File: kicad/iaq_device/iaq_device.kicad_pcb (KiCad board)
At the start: 2 copper layers, 78.2 x 43.2 mm, 18 parts, among them J1 External Pins, SW1 B3S-1000, SW2 CO2 CAL, U2 PMS7003, U3 SSD1306, U4 BME280, U5 MH-Z19, U6 SGP30, U7 TSL2561T

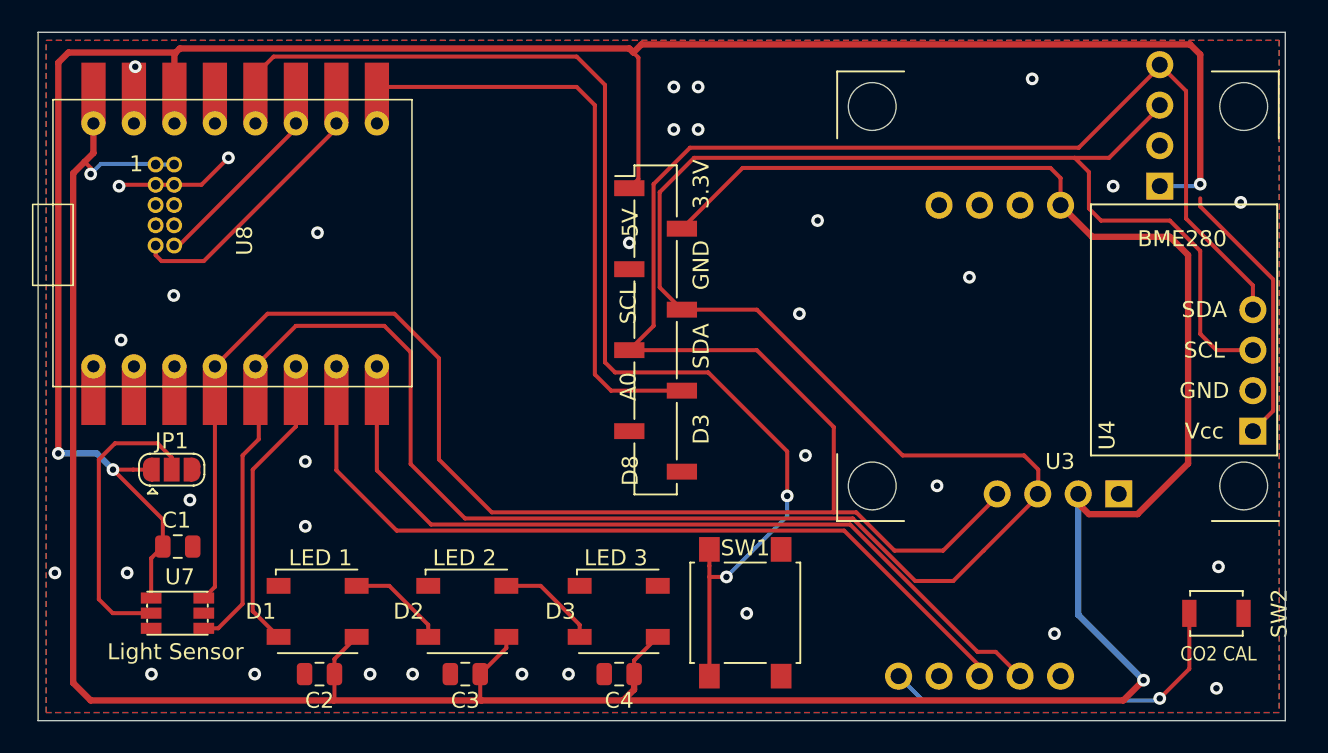
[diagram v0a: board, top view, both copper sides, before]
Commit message: v2.0 of the C3 PCB files
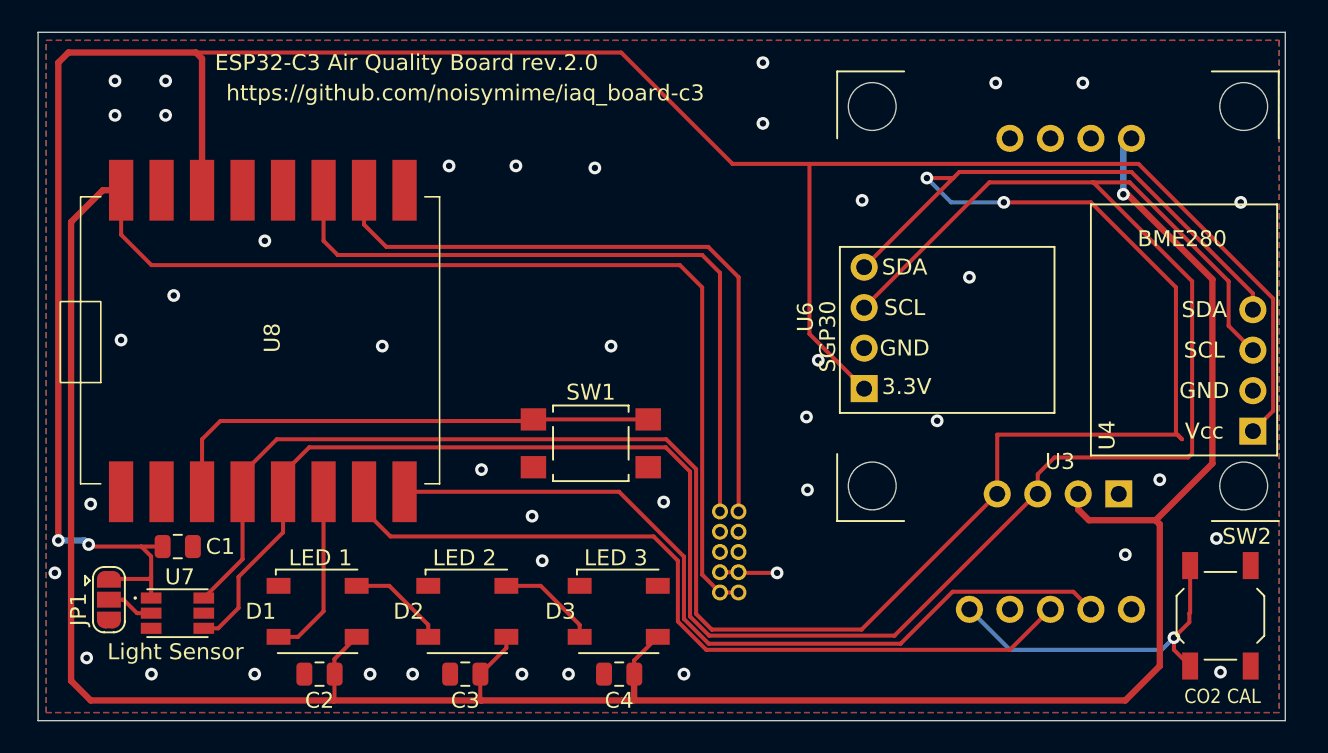
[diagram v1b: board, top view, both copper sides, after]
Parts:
- removed J1: External Pins, Connector_PinSocket_2.54mm:PinSocket_1x08_P2.54mm_Vertical_SMD_Pin1Left
- SW1: value B3S-1000 -> SEL; footprint Nikolay Library:SW_SPST_B3S-1000 -> Button_Switch_SMD:SW_SPST_TL3305B
- SW2: footprint Button_Switch_SMD:SW_SPST_B3U-1000P -> Button_Switch_SMD:SW_SPST_TL3342
- U6: moved to F.Cu
- moved U6 22.5 mm to (150.6, 96.3), turned to 180 degrees
- moved SW1 14.4 mm to (133.5, 99.7), turned to 0 degrees
- moved JP1 9.06 mm to (103.3, 109.5), turned to -90 degrees
- moved U8 6.34 mm to (101.5, 102.2)
- moved U5 6.11 mm to (167.4, 110.1)
- moved U2 0.76 mm to (124.5, 96.0), turned to 0 degrees
- moved SW2 0.29 mm to (173.0, 110.5), turned to -90 degrees
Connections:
- SW1 pad 1: Net-(U8-0) -> Net-(U8-7)
- U8 pad 4: unconnected-(U8-6-Pad4) -> D6
- U8 pad 6: unconnected-(U8-7-Pad6) -> Net-(U8-7)
- U8 pad 9: Net-(U8-0) -> unconnected-(U8-3-Pad9)
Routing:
- net Net-(U8-0): track 73.9 -> 0.00 mm, vias 2 -> 0
- net A0: track 37.1 -> 0.00 mm
- net PMS_SET: track 11.8 -> 43.8 mm
- net Net-(U8-7): track 0.00 -> 31.8 mm
- net SCL: track 170.2 -> 138.8 mm
- net PMS_RX: track 15.9 -> 41.7 mm
- net +5V: track 196.5 -> 221.8 mm, vias 2 -> 1
- net Net-(JP1-C): track 18.5 -> 3.00 mm
- net SDA: track 158.9 -> 147.1 mm, vias 0 -> 2
- net +3V3: track 152.2 -> 158.9 mm, vias 3 -> 2
- net LED_D: track 17.0 -> 11.0 mm
- net GND: track 7.74 -> 3.62 mm, vias 34 -> 42
- net Net-(U5-CAL): track 23.2 -> 21.3 mm
- net MH_TX: track 50.4 -> 51.1 mm
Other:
- rule solder_mask_min_width: 0.25 -> 0.2
- board text added: "ESP32-C3 Air Quality Board rev.2.0"
- board text removed: "1"
- board text removed: "3.3V"
- board text removed: "5V"
- board text removed: "A0"
- board text removed: "D3"
- board text removed: "D8"
- board text removed: "ESP32-C3 Air Quality Board rev.1.0"
- board text removed: "GND"
- board text removed: "SCL"
